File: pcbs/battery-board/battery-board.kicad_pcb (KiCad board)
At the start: 2 copper layers, 98 x 160 mm, 12 parts, among them J1 Conn_01x02, J2 Conn_01x02

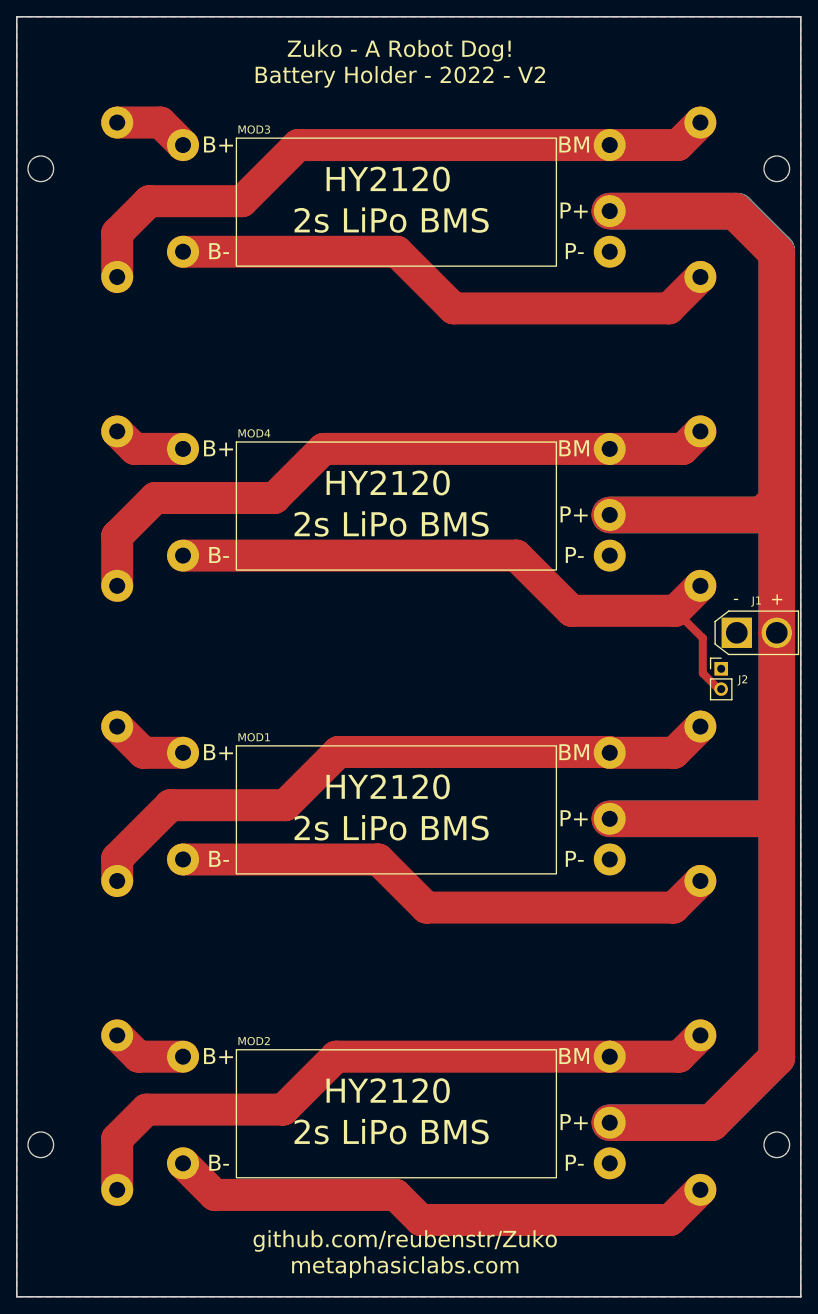
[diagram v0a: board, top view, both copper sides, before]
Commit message: pcb update
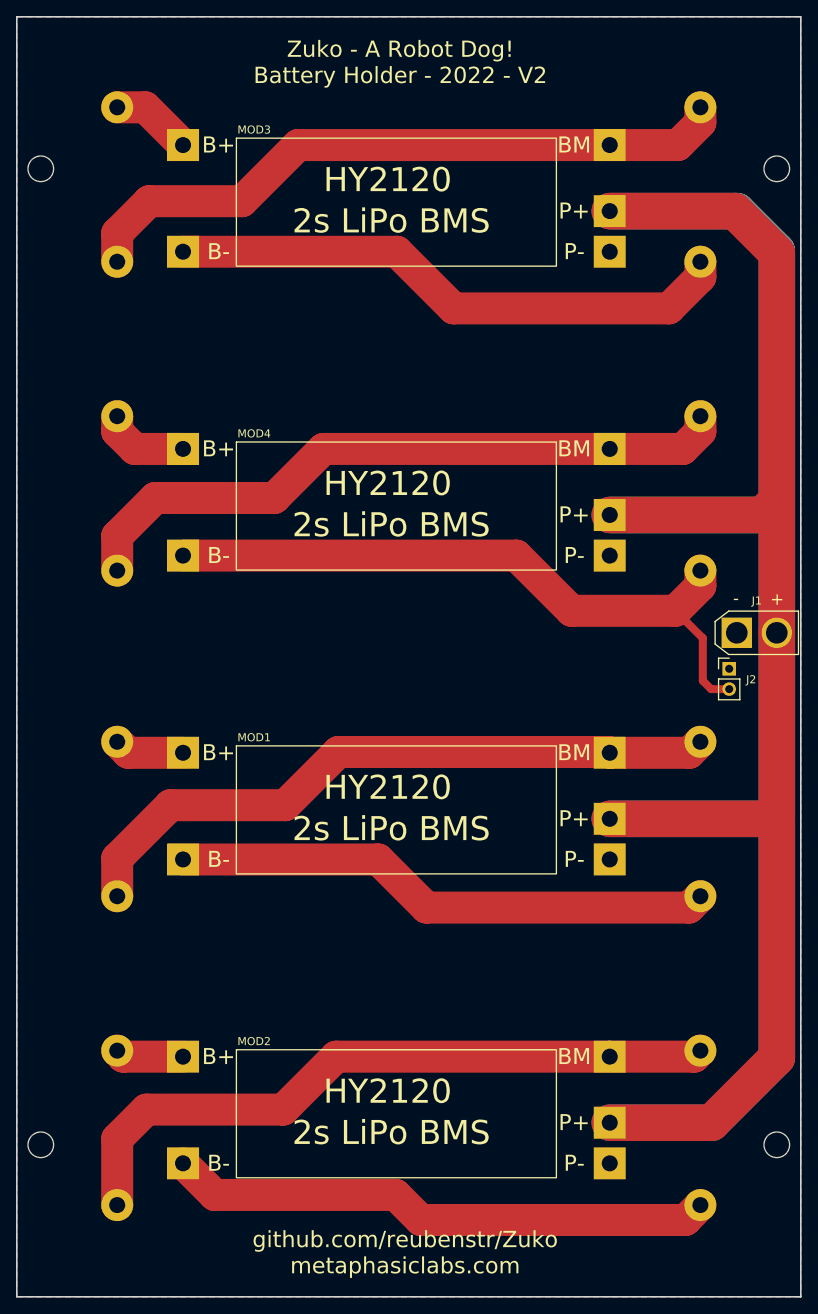
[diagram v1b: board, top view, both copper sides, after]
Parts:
- moved BH1 1.91 mm to (49.0, 80.4)
- moved BH2 1.91 mm to (49.0, 1.09)
- moved J2 1.00 mm to (89.0, 81.5)
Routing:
- net Net-(BH2-Pad4): track 82.7 -> 84.6 mm
- net Net-(BH2-Pad6): track 9.14 -> 11.0 mm
- net Net-(BH2-Pad2): track 69.2 -> 71.1 mm
- net Net-(BH1-Pad3): track 84.6 -> 85.7 mm
- net Net-(BH1-Pad1): track 82.6 -> 83.7 mm
- net Net-(BH1-Pad2): track 68.5 -> 67.8 mm
- net Net-(BH1-Pad8): track 9.59 -> 8.80 mm
- net Net-(BH1-Pad6): track 9.33 -> 8.54 mm
- net Net-(BH1-Pad4): track 69.2 -> 68.4 mm
- net Net-(BH2-Pad8): track 9.39 -> 10.2 mm
